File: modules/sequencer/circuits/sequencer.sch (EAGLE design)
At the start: 56 parts, among them IC2 LM324N

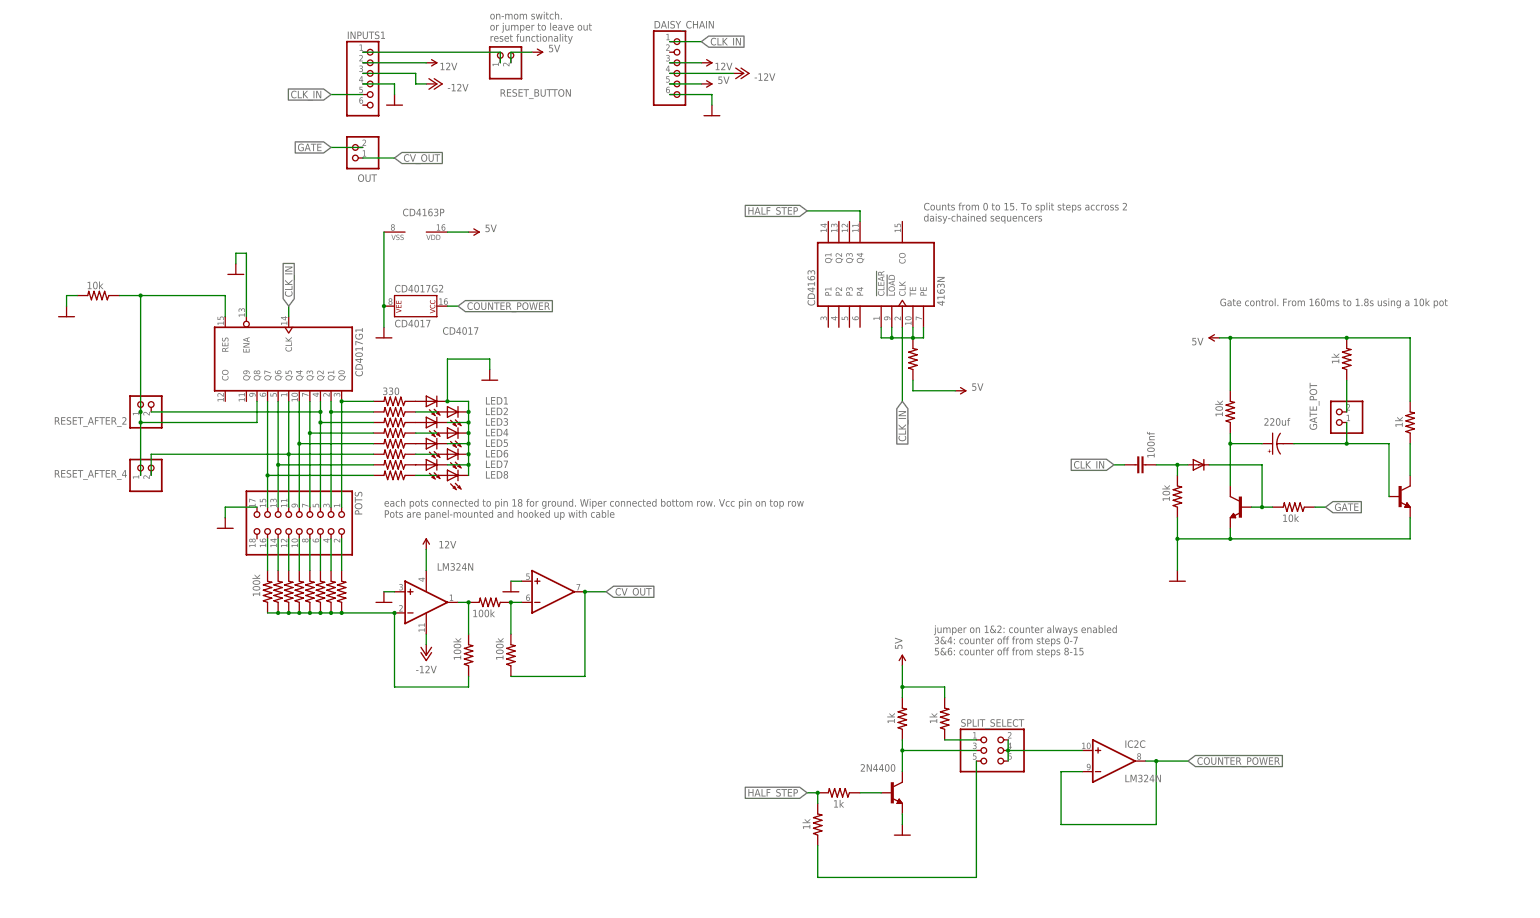
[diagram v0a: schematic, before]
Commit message: Seq board
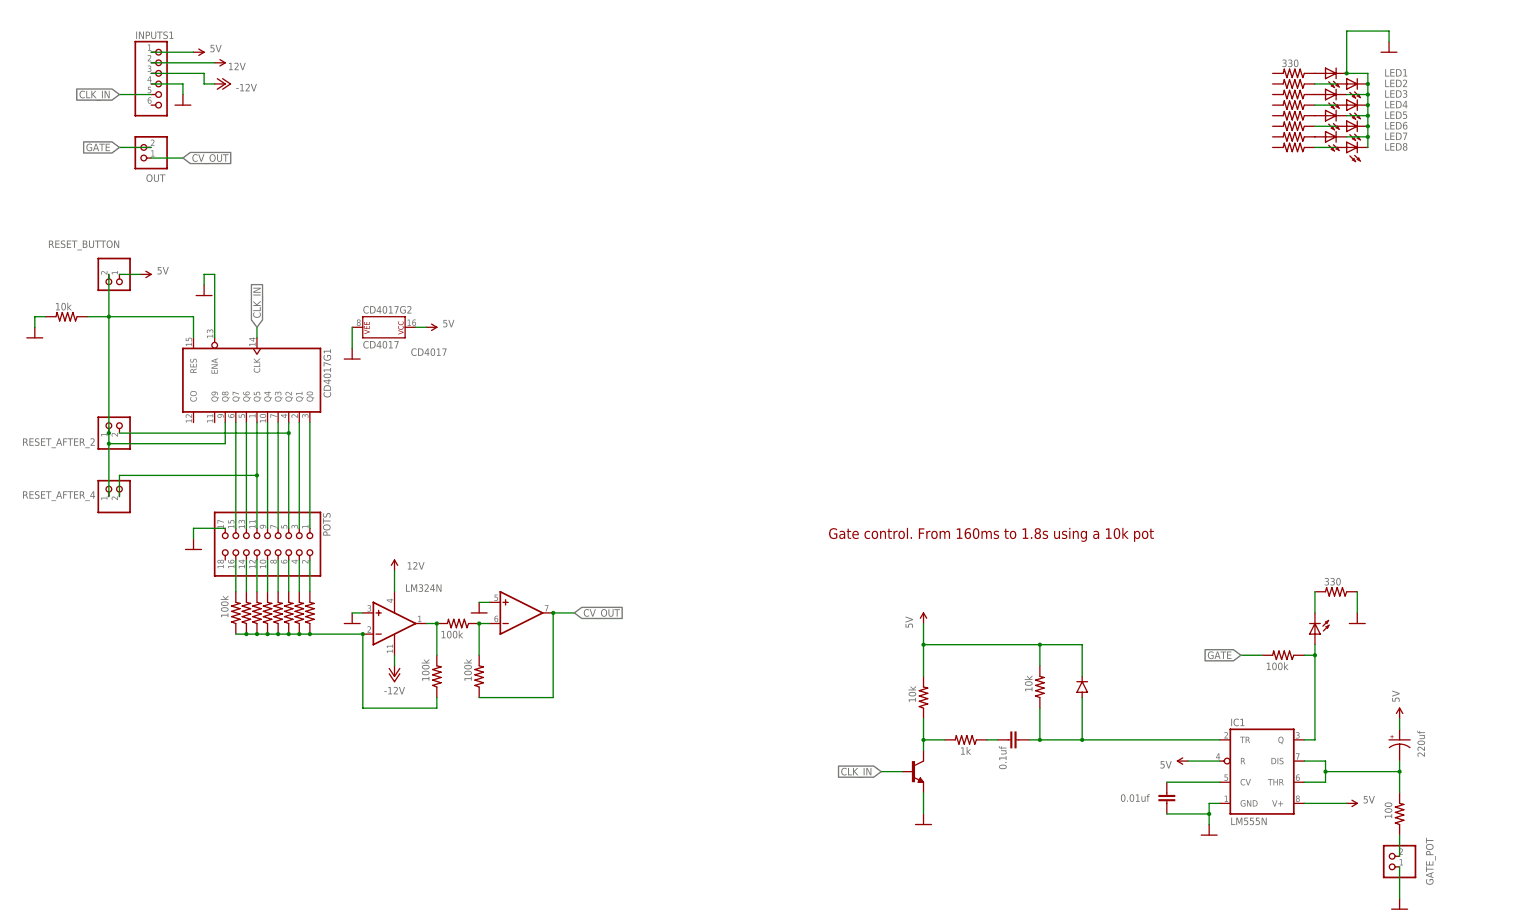
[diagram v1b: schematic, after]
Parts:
- removed 1K, 1K2: 1k, adafruit:R-US_0207/12
- removed 2N1, 2N4400: (no value), transistor-neu-to92:2N4401-NPN-TO92-EBC
- removed C3: 100nf, rcl:C-EU025-024X044
- removed CD4163: 4163N, 40xx:4163N
- removed DAISY_CHAIN: (no value), pinhead:PINHD-1X6
- removed R24, R25: 10k, adafruit:R-US_0207/12
- removed SPLIT_SELECT: (no value), pinhead:PINHD-2X3
- added C1: 0.01uf, rcl:C-EU025-024X044
- added C4: 0.1uf, rcl:C-EU025-024X044
- added IC1: LM555N, adafruit:LM555N
- added LED9: (no value), adafruit:LED5MM
- 1K1: value 1k -> 100k
- 1K4: value 1k -> 10k
- D1: device adafruit:1N4004 -> diode:1N4004
- R21: value 100k -> 100
- R23: value 1k -> 330
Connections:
- removed net COUNTER_POWER: CD4017G2.P$V+, IC2C.-IN, IC2C.OUT
- removed net HALF_STEP: 1K1.2, CD4163G$1.Q4, R23.2
- removed net N$37: IC2C.+IN, SPLIT_SELECT.2, SPLIT_SELECT.4, SPLIT_SELECT.6
- removed net N$38: 1K2.1, SPLIT_SELECT.1
- removed net N$39: 2N2.C, C2.+, R25.1
- removed net N$40: 1K3.1, 2N1.C
- removed net N$41: 1K4.1, GATE_POT.2
- removed net N$42: 2N1.B, C2.-, GATE_POT.1
- removed net RESET: CD4163G$1.!CLEAR, CD4163G$1.!LOAD, CD4163G$1.PE, CD4163G$1.TE, R21.2
- new net N$33: C4.1, D1.A, IC1.TR, R20.1
- new net N$34: C1.1, IC1.CV
- net -12V: no longer DAISY_CHAIN.4
- net 12V: no longer DAISY_CHAIN.3
- net 5V: now also C2.+, CD4017G2.P$V+, D1.C, IC1.R, IC1.V+, INPUTS1.1, R20.2, RESET_BUTTON.1; no longer 1K.2, 1K2.2, 1K3.2, CD4163P.VDD, DAISY_CHAIN.5, R21.1, R25.2, RESET_BUTTON.2
- net CLK_IN: now also 2N2.B; no longer C3.1, CD4163G$1.CLK, DAISY_CHAIN.1
- net GATE: now also 1K1.2; no longer R24.1
- net GND: now also C1.2, GATE_POT.1, IC1.GND, R23.1; no longer 2N1.E, 2N4400.E, CD4163P.VSS, DAISY_CHAIN.6, R20.1
- net N$1: now also RESET_BUTTON.2
- net N$10: no longer R19.2
- net N$2: now also 1K3.1, C4.2; no longer C3.2, D1.A, R20.2
- net N$3: no longer R1.2
- net N$30: now also LED9.C, R23.2; no longer 1K.1, 2N4400.C, SPLIT_SELECT.3
- net N$31: now also GATE_POT.2, R21.1; no longer 2N4400.B, R23.1
- net N$32: now also 1K3.2, 1K4.1, 2N2.C; no longer INPUTS1.1, RESET_BUTTON.1
- net N$35: now also C2.-, IC1.DIS, IC1.THR, R21.2; no longer 2N2.B, D1.C, R24.2
- net N$36: now also IC1.Q, LED9.A; no longer SPLIT_SELECT.5
- net N$4: no longer R13.2
- net N$5: no longer R14.2
- net N$6: no longer R15.2
- net N$7: no longer R16.2
- net N$8: no longer R17.2
- net N$9: no longer R18.2
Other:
- note added: "CV out will not be within the full range of 5V because of the output of the 4017. Ideally, everything would be powered from 12v and CV would be attenuated proportionally with the voltage measured before the POTs"
- note added: "differentiator"
- note added: "pulse generator"
- note added: "signal inverter"
- note added: "status led and ouput"
- note removed: "Counts from 0 to 15. To split steps accross 2 daisy-chained sequencers"
- note removed: "jumper on 1&2: counter always enabled 3&4: counter off from steps 0-7 5&6: counter off from steps 8-15"
- note removed: "on-mom switch. or jumper to leave out reset functionality"
- moved on the sheet: CD4017G1, CD4017G2, GATE_POT, INPUTS1, LED1, LED2, LED3, LED4, LED5, LED6, LED7, LED8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
